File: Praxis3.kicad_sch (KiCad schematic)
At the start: 9 parts, among them IC60 HCF4094YM013TR, IC61 HCF4094YM013TR, SW60 MSS3-V-T/R, SW61 B3U-3100P, U2 TPL5010, U60 LM555xM

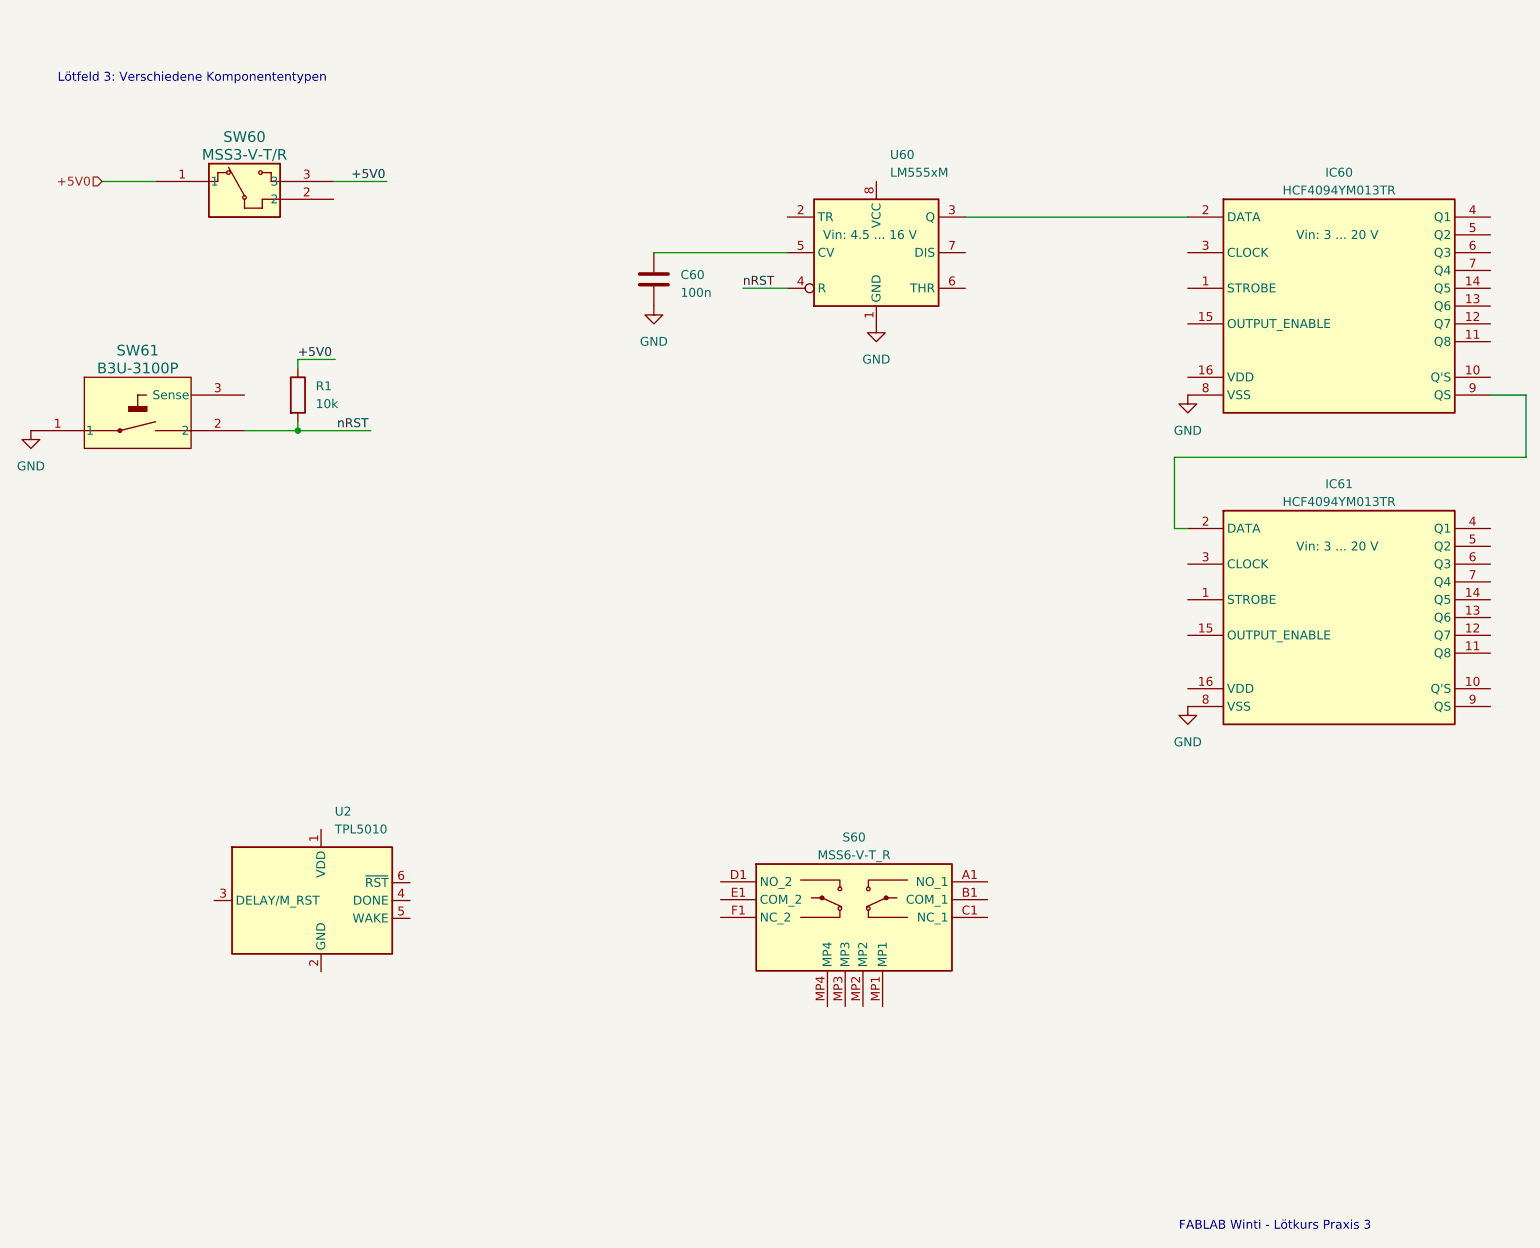
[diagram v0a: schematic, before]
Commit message: continued
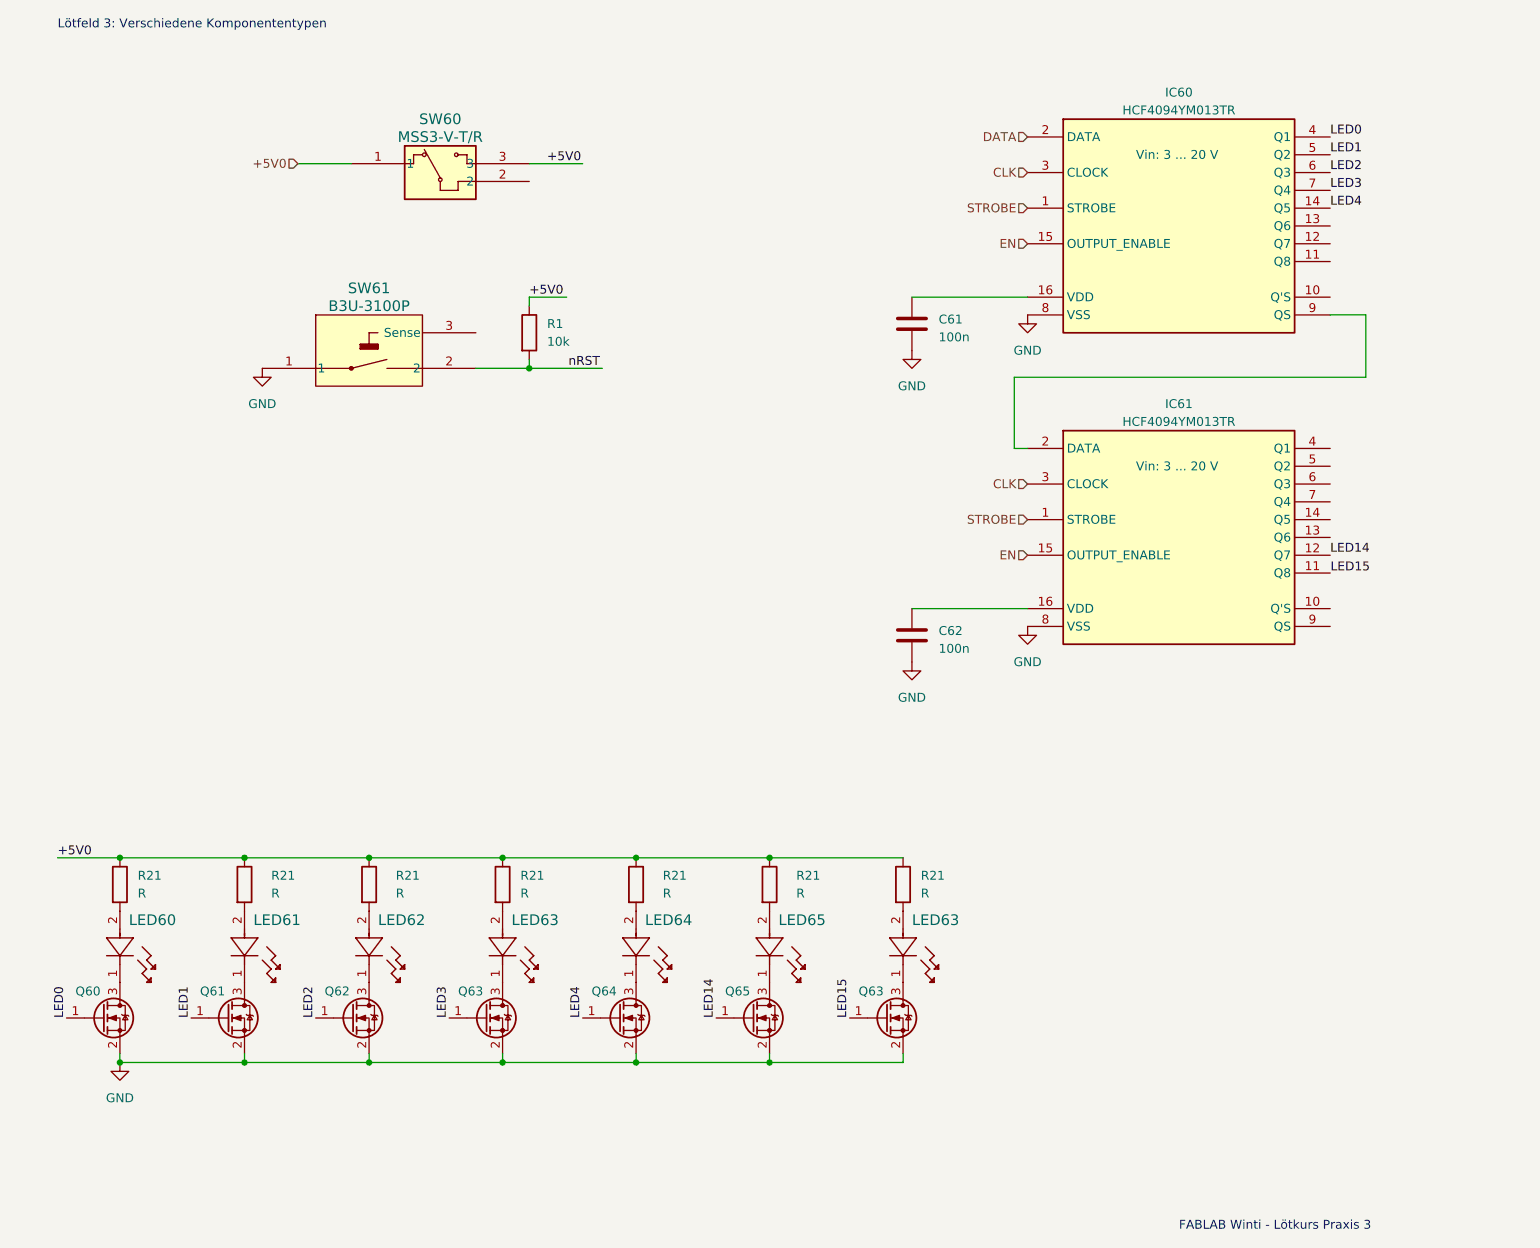
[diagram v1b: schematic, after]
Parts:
- removed C60: 100n, Capacitor_SMD:C_1206_3216Metric, symbol Device:C
- removed S60: MSS6-V-T_R, NiksKiCadLibrary:MSS6VTR, symbol NiksKiCadLibrary:MSS6-V-T_R
- removed U2: TPL5010, Package_TO_SOT_SMD:SOT-23-6, symbol Timer:TPL5010
- removed U60: LM555xM, Package_SO:SOIC-8_3.9x4.9mm_P1.27mm, symbol NiksKiCadLibrary:LM555xM
- added C61, C62: 100n, Capacitor_SMD:C_1206_3216Metric, symbol Device:C
- added LED60, LED61, LED62, LED63 (x2), LED64, LED65: SML-LX1206SIC-TR, FabLabWintiLibrary:LED_SML-LX1206SIC-TR_LUM, symbol FabLabWintiLibrary:SML-LX1206SIC-TR
- added Q60, Q61, Q62, Q63 (x2), Q64, Q65: 2N7002, Package_TO_SOT_SMD:SOT-23, symbol Transistor_FET:2N7002
- added R21 (x7): R, Resistor_SMD:R_1206_3216Metric, symbol Device:R
- SW61: footprint SW_B3U-3100P_OMR -> NiksKiCadLibrary:SW_B3U-3100P_OMR
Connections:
- net +5V0: now also R21.1, R21.1, R21.1, R21.1, R21.1, R21.1, R21.1
- net GND: now also C61.2, C62.2, Q60.2 (S), Q61.2 (S), Q62.2 (S), Q63.2 (S), Q63.2 (S), Q64.2 (S), Q65.2 (S)
- net STROBE: now reaches IC60.1 (STROBE)
- net STROBE: now also IC61.1 (STROBE)
- net LED4: now reaches IC60.14 (Q5)
- net LED4: now also Q64.1 (G)
- net EN: now reaches IC60.15 (OUTPUT_ENABLE)
- net EN: now also IC61.15 (OUTPUT_ENABLE)
- net at IC60.16 (VDD): now also C61.1
- net DATA: now reaches IC60.2 (DATA)
- net CLK: now reaches IC60.3 (CLOCK)
- net CLK: now also IC61.3 (CLOCK)
- net LED0: now reaches IC60.4 (Q1)
- net LED0: now also Q60.1 (G)
- net LED1: now reaches IC60.5 (Q2)
- net LED1: now also Q61.1 (G)
- net LED2: now reaches IC60.6 (Q3)
- net LED2: now also Q62.1 (G)
- net LED3: now reaches IC60.7 (Q4)
- net LED3: now also Q63.1 (G)
- net LED14: now reaches IC61.12 (Q7)
- net LED14: now also Q65.1 (G)
- net at IC61.16 (VDD): now also C62.1
- new net: LED60.2, R21.2
- new net: LED63.1, Q63.3 (D) (x2)
- new net: LED63.2, R21.2 (x2)
- new net: LED64.1, Q64.3 (D)
- new net: LED65.1, Q65.3 (D)
- new net: LED65.2, R21.2
- new net: LED64.2, R21.2
- new net: LED62.1, Q62.3 (D)
- new net: LED61.1, Q61.3 (D)
- new net: LED61.2, R21.2
- new net: LED60.1, Q60.3 (D)
- new net: LED62.2, R21.2
- new net LED15: Q63.1 (G)
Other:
- moved on the sheet: IC60, IC61, R1, SW60, SW61
